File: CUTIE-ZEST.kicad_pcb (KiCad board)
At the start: 4 copper layers, 78.5 x 78.5 mm, 65 parts, among them J1 TC2030, J2 U.FL, J3 U.FL, P1 ERM8-025-01-L-D-RA-K-TR, U1 TCAN334, U2 MCP98243, U3 ADP7158ACPZ-3.3-R7, U4 STM32G474CEUx, U5 AS179-92LF, U6 SX1262IMLTRT, U7 SN74LVC1G14DBV, U8 NEO-M8M, Y1 ECS-TXO-2520MV

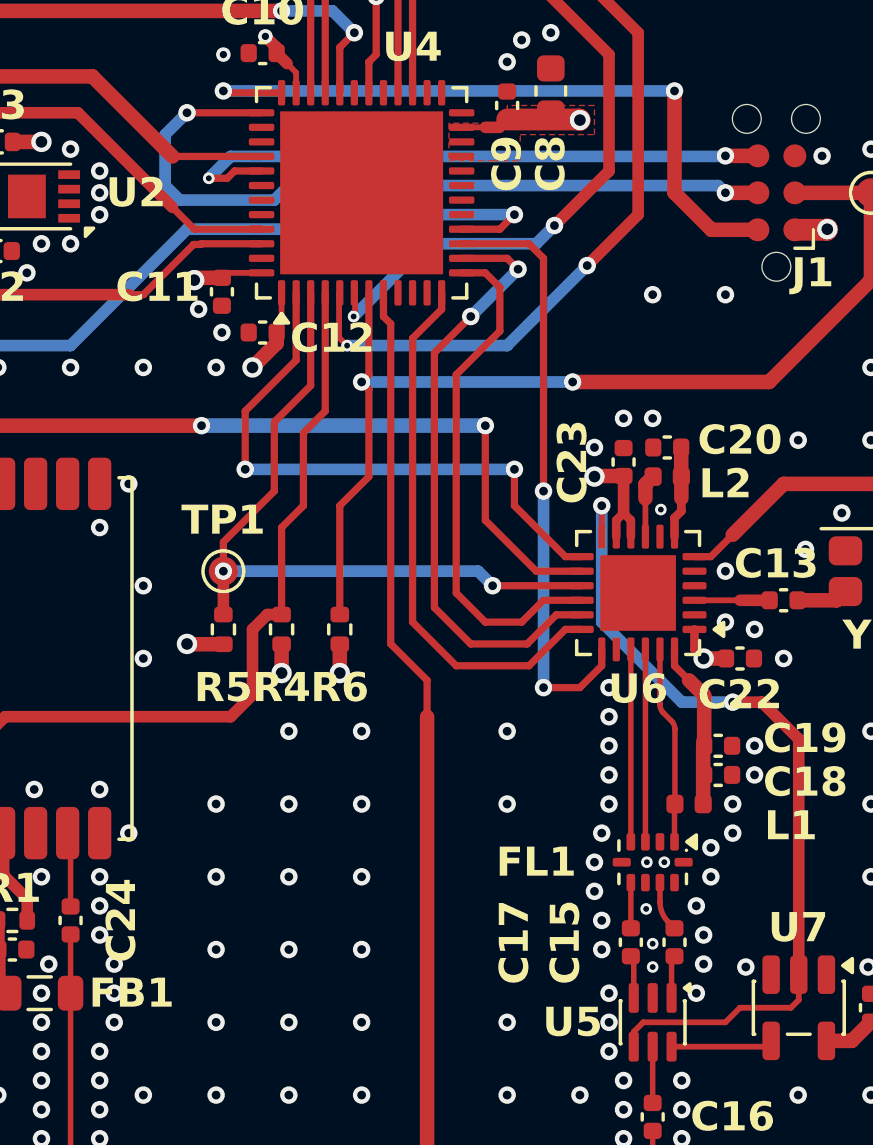
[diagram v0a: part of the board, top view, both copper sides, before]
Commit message: push for fab
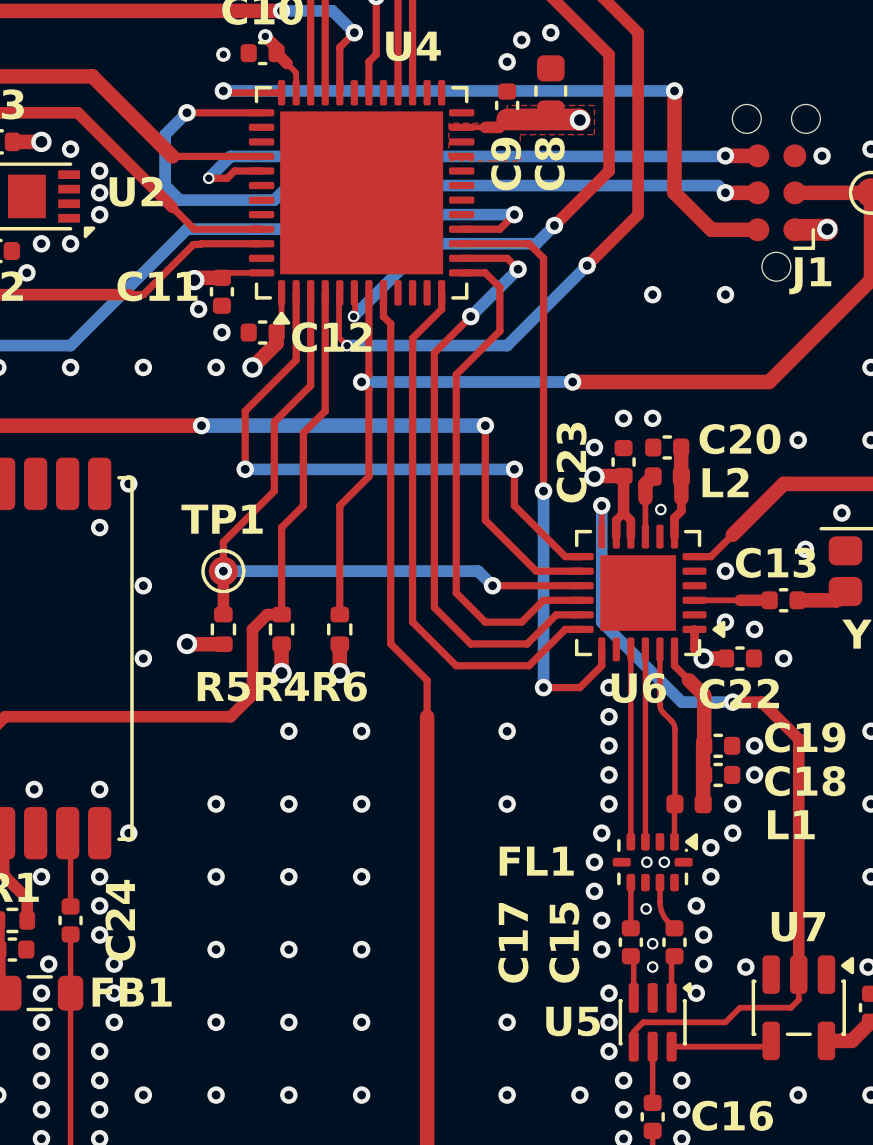
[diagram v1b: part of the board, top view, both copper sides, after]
